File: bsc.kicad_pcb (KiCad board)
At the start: 2 copper layers, 120 x 72 mm, 155 parts, among them IC1 ILD217T, IC2 ILD217T, J1 AVR-ISP-6, J2 Prog, J3 U0TXD silent, J4 Boot, K1 TIANBO-HJR-4102-L, K2 TIANBO-HJR-4102-L, K3 TIANBO-HJR-4102-L, K4 TIANBO-HJR-4102-L, K5 TIANBO-HJR-4102-L, K6 TIANBO-HJR-4102-L, K7 TIANBO-HJR-4102-L, K8 AQY210S, Q1 BSS138, Q10 BC846, Q11 BC846, Q2 BSS138, Q3 BSS138, Q4 BSS138, Q5 BSS138, Q6 BSS138, Q7 BSS138, Q8 BC846, Q9 BC846, U1 LMO78_03-0.5, U10 74HC595, U11 74HC14, U12 74HC165, U2 ESP32WROOM32E16, U3 ATtiny24A-SS, U4 ADuM1201AR, U5 ADuM1201AR, U6 ADuM1201AR, U7 SN65HVD234, U8 SP3485EN, U9 SP3485EN, X1 Conn_S2, X2 Conn_S1, X3 Conn_DI, X4 Conn_SV, X5 Conn_Rel2, X6 Conn_Rel1

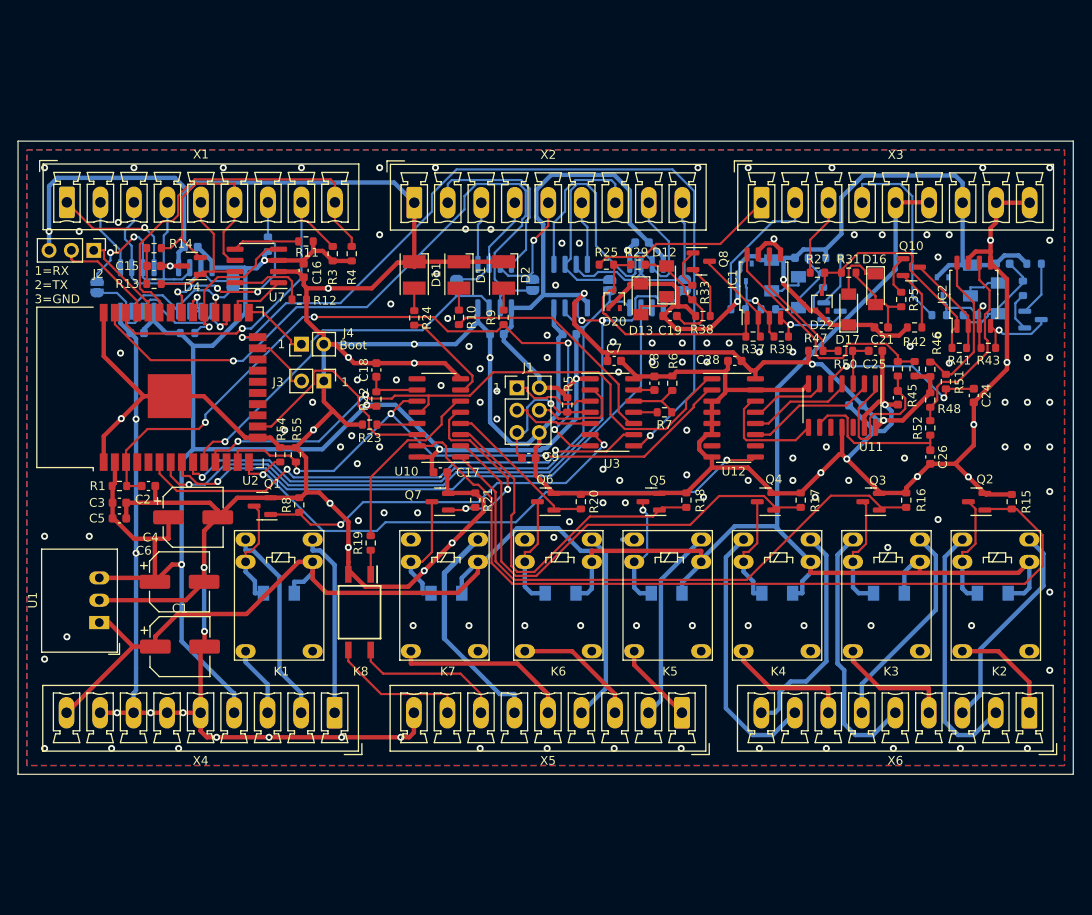
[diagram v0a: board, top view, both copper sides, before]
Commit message: Redesign PCB
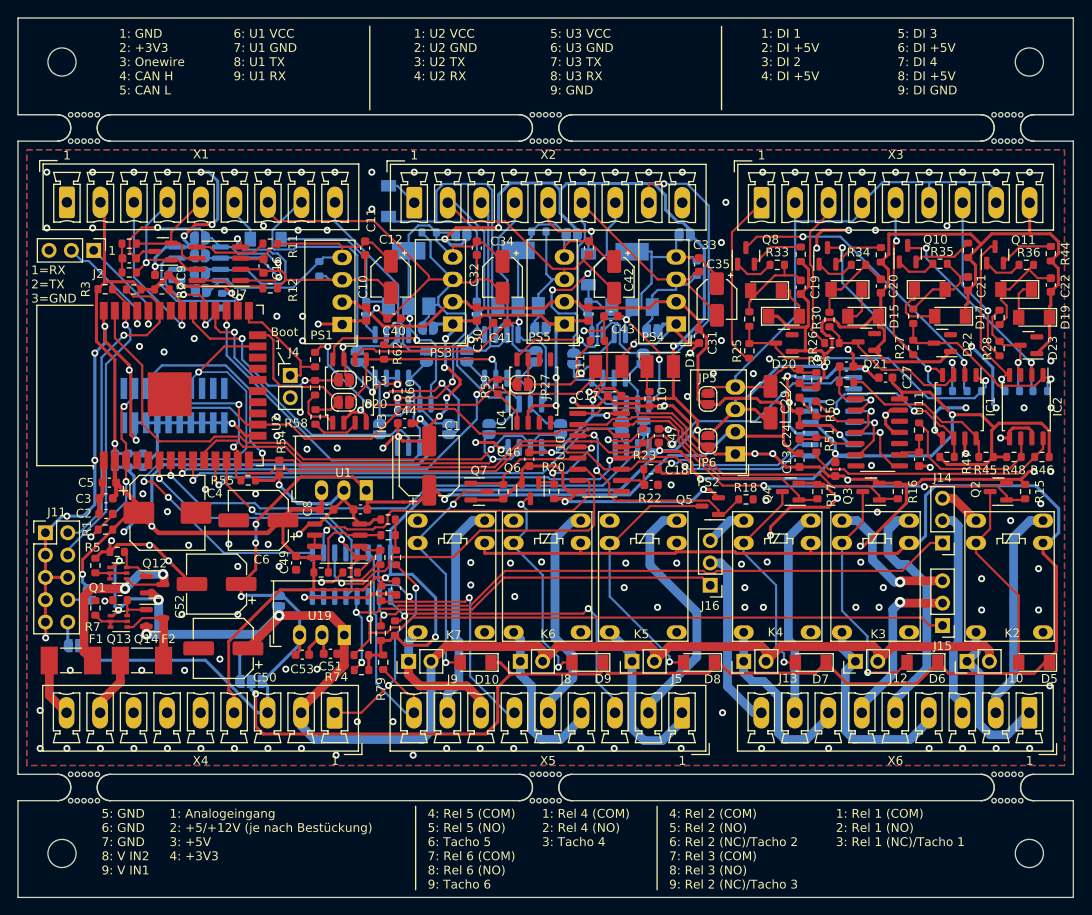
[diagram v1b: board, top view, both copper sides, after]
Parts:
- removed J3: U0TXD silent, Connector_PinHeader_2.54mm:PinHeader_1x02_P2.54mm_Vertical
- removed K1: TIANBO-HJR-4102-L, Relay_THT:Relay_SPDT_HJR-4102
- removed K8: AQY210S, SamacSys_Parts:SOP254P962X275-4N
- removed R9: 180R, Resistor_SMD:R_0603_1608Metric
- removed U3: ATtiny24A-SS, Package_SO:SOIC-14_3.9x8.7mm_P1.27mm
- added C29: 22µ, Capacitor_SMD:CP_Elec_4x5.8, F.Cu at (115.6, 59.7)
- added C30: 100n, Capacitor_SMD:C_0603_1608Metric, F.Cu at (82.2, 49.7)
- added C31: 100n, Capacitor_SMD:C_0603_1608Metric, F.Cu at (107.4, 52.2)
- added C32: 100n, Capacitor_SMD:C_0603_1608Metric, F.Cu at (82.2, 42.2)
- added C33: 100n, Capacitor_SMD:C_0603_1608Metric, F.Cu at (107.4, 44.1)
- added C34: 22µ, Capacitor_SMD:CP_Elec_4x5.8, F.Cu at (85.1, 45.5)
- added C35: 22µ, Capacitor_SMD:CP_Elec_4x5.8, F.Cu at (109.5, 48.0)
- added C36: 100n, Capacitor_SMD:C_0603_1608Metric, B.Cu at (69.6, 49.0)
- added C37: 100n, Capacitor_SMD:C_0603_1608Metric, B.Cu at (94.9, 49.0)
- added C38: 100n, Capacitor_SMD:C_0603_1608Metric, F.Cu at (94.9, 49.7)
- added C39: 100n, Capacitor_SMD:C_0603_1608Metric, F.Cu at (94.9, 42.1)
- added C40: 100n, Capacitor_SMD:C_0603_1608Metric, F.Cu at (72.8, 50.2)
- added C41: 100n, Capacitor_SMD:C_0603_1608Metric, F.Cu at (84.8, 50.7)
- added C42: 22µ, Capacitor_SMD:CP_Elec_4x5.8, F.Cu at (97.8, 45.5)
- added C43: 100n, Capacitor_SMD:C_0603_1608Metric, F.Cu at (97.4, 49.9)
- added C44: 100n, Capacitor_SMD:C_0603_1608Metric, F.Cu at (74.0, 62.1)
- added C45: 100n, Capacitor_SMD:C_0603_1608Metric, B.Cu at (82.2, 49.0)
- added C46: 100n, Capacitor_SMD:C_0603_1608Metric, F.Cu at (88.1, 66.2)
- added C47: 100n, Capacitor_SMD:C_0603_1608Metric, F.Cu at (102.9, 63.5)
- added C48: 100n, Capacitor_SMD:C_0603_1608Metric, B.Cu at (42.5, 66.3)
- added C49: 100n, Capacitor_SMD:C_0603_1608Metric, F.Cu at (61.6, 78.0)
- added C50: 100µ, Capacitor_SMD:CP_Elec_6.3x5.9, F.Cu at (53.3, 87.7)
- added C51: 100n, Capacitor_SMD:C_0603_1608Metric, F.Cu at (65.5, 88.3)
- added C52: 100µ, Capacitor_SMD:CP_Elec_6.3x5.9, F.Cu at (52.6, 80.4)
- added C53: 100n, Capacitor_SMD:C_0603_1608Metric, F.Cu at (62.3, 88.4)
- added C54: 100n, Capacitor_SMD:C_0603_1608Metric, B.Cu at (41.0, 66.3)
- added C55: 100n, Capacitor_SMD:C_0603_1608Metric, B.Cu at (44.2, 66.3)
- added C60: 100n, Capacitor_SMD:C_0603_1608Metric, F.Cu at (73.0, 80.8)
- added D24: LL4148, Diode_SMD:D_MiniMELF, B.Cu at (72.1, 36.8)
- added F1: BELFUSE, Fuse:Fuse_0679H, F.Cu at (36.0, 89.1)
- added F2: BELFUSE, Fuse:Fuse_0679H, F.Cu at (44.1, 89.1)
- added H1: MountingHole, MountingHole:MountingHole_3.2mm_M3, F.Cu at (35.0, 21.0)
- added H2: MountingHole, MountingHole:MountingHole_3.2mm_M3, F.Cu at (145.0, 21.0)
- added H3: MountingHole, MountingHole:MountingHole_3.2mm_M3, F.Cu at (145.0, 111.0)
- added H4: MountingHole, MountingHole:MountingHole_3.2mm_M3, F.Cu at (35.0, 111.0)
- added IC3: ILD217T, Package_SO:SOIC-8_5.23x5.23mm_P1.27mm, F.Cu at (67.7, 58.4)
- added IC4: ILD217T, Package_SO:SOIC-8_5.23x5.23mm_P1.27mm, F.Cu at (88.6, 58.4)
- added J10: JP_REL1_COM_12V, Connector_PinHeader_2.54mm:PinHeader_1x02_P2.54mm_Vertical, F.Cu at (137.9, 89.2)
- added J11: Conn_Extension, Connector_PinHeader_2.54mm:PinHeader_2x05_P2.54mm_Vertical, F.Cu at (33.1, 74.5)
- added J12: JP_REL2_COM_12V, Connector_PinHeader_2.54mm:PinHeader_1x02_P2.54mm_Vertical, F.Cu at (125.2, 89.2)
- added J13: JP_REL3_COM_12V, Connector_PinHeader_2.54mm:PinHeader_1x02_P2.54mm_Vertical, F.Cu at (112.5, 89.2)
- added J14: Conn_REL1, Connector_PinHeader_2.54mm:PinHeader_1x03_P2.54mm_Vertical, F.Cu at (135.1, 75.7)
- added J15: Conn_REL2, Connector_PinHeader_2.54mm:PinHeader_1x03_P2.54mm_Vertical, F.Cu at (135.1, 85.1)
- added J16: Conn_REL3, Connector_PinHeader_2.54mm:PinHeader_1x03_P2.54mm_Vertical, F.Cu at (108.7, 80.5)
- added J5: JP_REL4_COM_12V, Connector_PinHeader_2.54mm:PinHeader_1x02_P2.54mm_Vertical, F.Cu at (99.8, 89.2)
- added J8: JP_REL5_COM_12V, Connector_PinHeader_2.54mm:PinHeader_1x02_P2.54mm_Vertical, F.Cu at (87.1, 89.2)
- added J9: JP_REL6_COM_12V, Connector_PinHeader_2.54mm:PinHeader_1x02_P2.54mm_Vertical, F.Cu at (74.4, 89.2)
- added JP10: JP_U1_TX_TXS, Jumper:SolderJumper-2_P1.3mm_Open_RoundedPad1.0x1.5mm, B.Cu at (71.1, 62.7)
- added JP11: JP_U1_RXS_RXO, Jumper:SolderJumper-2_P1.3mm_Open_RoundedPad1.0x1.5mm, B.Cu at (76.5, 54.5)
- added JP12: JP_U1_TXS_TXO, Jumper:SolderJumper-2_P1.3mm_Open_RoundedPad1.0x1.5mm, B.Cu at (68.6, 54.5)
- added JP13: JP_U1_TXEN_TXENS, Jumper:SolderJumper-2_P1.3mm_Open_RoundedPad1.0x1.5mm, F.Cu at (67.1, 57.1)
- added JP14: JP_U2_3V3_VCC, Jumper:SolderJumper-2_P1.3mm_Open_RoundedPad1.0x1.5mm, B.Cu at (93.0, 40.6)
- added JP15: JP_U2_GND_GNDS, Jumper:SolderJumper-2_P1.3mm_Open_RoundedPad1.0x1.5mm, B.Cu at (89.4, 51.3)
- added JP16: JP_U2_RX_RXS, Jumper:SolderJumper-2_P1.3mm_Open_RoundedPad1.0x1.5mm, B.Cu at (91.7, 62.7)
- added JP17: JP_U2_TX_TXS, Jumper:SolderJumper-2_P1.3mm_Open_RoundedPad1.0x1.5mm, B.Cu at (83.6, 62.7)
- added JP18: JP_U2_RXS_RXO, Jumper:SolderJumper-2_P1.3mm_Open_RoundedPad1.0x1.5mm, B.Cu at (88.9, 54.5)
- added JP19: JP_U2_TXS_TXO, Jumper:SolderJumper-2_P1.3mm_Open_RoundedPad1.0x1.5mm, B.Cu at (81.0, 54.5)
- added JP20: JP_U2_TXEN_TXENS, Jumper:SolderJumper-2_P1.3mm_Open_RoundedPad1.0x1.5mm, F.Cu at (67.1, 59.7)
- added JP21: JP_U3_3V3_VCC, Jumper:SolderJumper-2_P1.3mm_Open_RoundedPad1.0x1.5mm, B.Cu at (105.8, 40.6)
- added JP22: JP_U3_GND_GNDS, Jumper:SolderJumper-2_P1.3mm_Open_RoundedPad1.0x1.5mm, B.Cu at (102.1, 51.6)
- added JP23: JP_U3_RX_RXS, Jumper:SolderJumper-2_P1.3mm_Open_RoundedPad1.0x1.5mm, B.Cu at (101.2, 62.4)
- added JP24: JP_U3_TX_TXS, Jumper:SolderJumper-2_P1.3mm_Open_RoundedPad1.0x1.5mm, B.Cu at (98.7, 62.4)
- added JP25: JP_U3_RXS_RXO, Jumper:SolderJumper-2_P1.3mm_Open_RoundedPad1.0x1.5mm, B.Cu at (101.1, 54.7)
- added JP26: JP_U3_TXS_TXO, Jumper:SolderJumper-2_P1.3mm_Open_RoundedPad1.0x1.5mm, B.Cu at (93.2, 54.7)
- added JP27: JP_U3_TXEN_TXENS, Jumper:SolderJumper-2_P1.3mm_Open_RoundedPad1.0x1.5mm, F.Cu at (87.4, 57.7)
- added JP28: 12V_5V, Jumper:SolderJumper-2_P1.3mm_Open_RoundedPad1.0x1.5mm, B.Cu at (59.6, 82.3)
- added JP29: JP_REL_VCC, Jumper:SolderJumper-3_P1.3mm_Open_RoundedPad1.0x1.5mm, B.Cu at (56.5, 91.4)
- added JP30: JP_EXT_5V, Jumper:SolderJumper-2_P1.3mm_Open_RoundedPad1.0x1.5mm, B.Cu at (36.4, 87.4)
- added JP31: JP_EXT_3V3, Jumper:SolderJumper-2_P1.3mm_Open_RoundedPad1.0x1.5mm, B.Cu at (38.1, 81.5)
- added JP7: JP_U1_3V3_VCC, Jumper:SolderJumper-2_P1.3mm_Open_RoundedPad1.0x1.5mm, B.Cu at (80.4, 40.6)
- added JP8: JP_U1_GND_GNDS, Jumper:SolderJumper-2_P1.3mm_Open_RoundedPad1.0x1.5mm, B.Cu at (76.6, 51.3)
- added JP9: JP_U1_RX_RXS, Jumper:SolderJumper-2_P1.3mm_Open_RoundedPad1.0x1.5mm, B.Cu at (79.0, 62.7)
- added PS1: 1S4E_0503S1U, custom_th:Converter_DCDC_GAPTEC_1S4E_S1U, F.Cu at (66.9, 50.9)
- added PS2: TEA 1-0505, Converter_DCDC:Converter_DCDC_Murata_MEE1SxxxxSC_THT, F.Cu at (111.6, 65.6)
- added PS3: 1S4E_0503S1U, custom_th:Converter_DCDC_GAPTEC_1S4E_S1U, F.Cu at (79.4, 50.8)
- added PS4: 1S4E_0503S1U, custom_th:Converter_DCDC_GAPTEC_1S4E_S1U, F.Cu at (104.8, 50.8)
- added PS5: 1S4E_0503S1U, custom_th:Converter_DCDC_GAPTEC_1S4E_S1U, F.Cu at (92.1, 50.8)
- added Q12: IRLML2244, Package_TO_SOT_SMD:SOT-23, F.Cu at (45.5, 80.4)
- added Q13: BC857BS, Package_TO_SOT_SMD:SOT-363_SC-70-6, F.Cu at (41.5, 84.6)
- added Q14: IRLML2244, Package_TO_SOT_SMD:SOT-23, F.Cu at (45.5, 84.2)
- added R56: n.b., Resistor_SMD:R_0603_1608Metric, F.Cu at (120.8, 57.1)
- added R57: 330R, Resistor_SMD:R_0603_1608Metric, F.Cu at (63.8, 58.0)
- added R58: 330R, Resistor_SMD:R_0603_1608Metric, F.Cu at (63.8, 61.4)
- added R59: 330R, Resistor_SMD:R_0603_1608Metric, F.Cu at (84.6, 57.9)
- added R60: 2k2, Resistor_SMD:R_0603_1608Metric, F.Cu at (73.2, 58.4)
- added R61: 2k2, Resistor_SMD:R_0603_1608Metric, F.Cu at (95.9, 52.7)
- added R62: 2k2, Resistor_SMD:R_0603_1608Metric, F.Cu at (71.6, 54.0)
- added R63: n.b., Resistor_SMD:R_0603_1608Metric, B.Cu at (76.7, 40.4)
- added R64: n.b., Resistor_SMD:R_0603_1608Metric, B.Cu at (107.2, 44.5)
- added R65: n.b., Resistor_SMD:R_0603_1608Metric, B.Cu at (89.2, 40.3)
- added R66: 10k, Resistor_SMD:R_0603_1608Metric, F.Cu at (73.0, 77.3)
- added R67: 2k4, Resistor_SMD:R_0603_1608Metric, F.Cu at (72.1, 73.0)
- added R68: 470R, Resistor_SMD:R_0603_1608Metric, F.Cu at (72.1, 74.8)
- added R69: 47k, Resistor_SMD:R_0603_1608Metric, F.Cu at (64.5, 79.0)
- added R70: 20k, Resistor_SMD:R_0603_1608Metric, F.Cu at (67.8, 79.0)
- added R71: 10k, Resistor_SMD:R_0603_1608Metric, F.Cu at (71.2, 77.3)
- added R74: 4k7, Resistor_SMD:R_0603_1608Metric, F.Cu at (69.1, 90.1)
- added R75: 4k7, Resistor_SMD:R_0603_1608Metric, F.Cu at (69.0, 88.4)
- added R76: 4k7, Resistor_SMD:R_0603_1608Metric, F.Cu at (71.2, 86.0)
- added R77: 4k7, Resistor_SMD:R_0603_1608Metric, F.Cu at (72.9, 85.4)
- added R78: 4k7, Resistor_SMD:R_0603_1608Metric, F.Cu at (71.3, 81.4)
- added R79: 4k7, Resistor_SMD:R_0603_1608Metric, F.Cu at (71.5, 89.3)
- added U13: ADuM1201AR, Package_SO:SOIC-8_3.9x4.9mm_P1.27mm, B.Cu at (50.5, 43.9)
- added U14: NCP1117-3.3_SOT223, Package_TO_SOT_SMD:SOT-223-3_TabPin2, B.Cu at (74.4, 45.6)
- added U15: NCP1117-3.3_SOT223, Package_TO_SOT_SMD:SOT-223-3_TabPin2, B.Cu at (99.8, 45.7)
- added U16: SP3485EN, Package_SO:SOIC-8_3.9x4.9mm_P1.27mm, B.Cu at (85.0, 54.5)
- added U17: NCP1117-3.3_SOT223, Package_TO_SOT_SMD:SOT-223-3_TabPin2, B.Cu at (86.9, 45.6)
- added U18: TS912, Package_SO:SO-8_3.9x4.9mm_P1.27mm, F.Cu at (66.3, 75.4)
- added U19: LMO78_05-0.5, custom_th:Converter_DCDC_RECOM_R-78E-1.0, F.Cu at (64.4, 83.6)
- added U20: HC 151, Package_SO:SOIC-16_3.9x9.9mm_P1.27mm, B.Cu at (67.9, 79.3)
- added mouse-bite-3mm-slot: VAL**, mouse_bites:mouse-bite-3mm-slot, F.Cu at (142.5, 28.5)
- added mouse-bite-3mm-slot: VAL**, mouse_bites:mouse-bite-3mm-slot, F.Cu at (142.5, 103.5)
- added mouse-bite-3mm-slot: VAL**, mouse_bites:mouse-bite-3mm-slot, F.Cu at (37.5, 103.5)
- added mouse-bite-3mm-slot: VAL**, mouse_bites:mouse-bite-3mm-slot, F.Cu at (37.5, 28.5)
- added mouse-bite-3mm-slot: VAL**, mouse_bites:mouse-bite-3mm-slot, F.Cu at (90.0, 103.5)
- added mouse-bite-3mm-slot: VAL**, mouse_bites:mouse-bite-3mm-slot, F.Cu at (90.0, 28.5)
- C1: value 10µ -> 100µ
- C10, C11, C13, C14, C20, C22, C27, D10, D14, D15, D18, D19, D5, D6, D7, D8, D9, Q11, Q9, R2, R26, R28, R30, R32, R34, R36, R40, R44: moved to F.Cu
- C12: value 100n -> 22µ; footprint Capacitor_SMD:C_0603_1608Metric -> Capacitor_SMD:CP_Elec_4x5.8; moved to F.Cu
- C15, C16, C5, C8: value 100nF -> 100n
- C4: value 22µ -> 470µ/6,3V; footprint Capacitor_SMD:CP_Elec_6.3x5.9 -> Capacitor_SMD:CP_Elec_8x10
- C6: value 22µ -> 100µ
- D2: value LED3 -> LL4148; footprint LED_SMD:LED_PLCC-2 -> Diode_SMD:D_MiniMELF; moved to B.Cu
- D20, D22: footprint Package_TO_SOT_SMD:SOT-323_SC-70 -> Package_TO_SOT_SMD:SOT-23
- D21, D23: footprint Package_TO_SOT_SMD:SOT-323_SC-70 -> Package_TO_SOT_SMD:SOT-23; moved to F.Cu
- J1: value AVR-ISP-6 -> Conn_JTAG_ESP; footprint Connector_PinHeader_2.54mm:PinHeader_2x03_P2.54mm_Vertical -> Connector_PinHeader_1.27mm:PinHeader_2x10_P1.27mm_Vertical_SMD; moved to B.Cu
- JP1: value O_U2RXD -> CAN_VCC
- JP2: value O_U2TXD -> CAN_GND
- JP3: value O_SU1RXD -> CAN_RC
- JP4: value O_SU1TXD -> CAN_TX
- JP5: value O_SU2RXD -> DI_VCC; moved to F.Cu
- JP6: value O_SU2TXD -> DI_GND; moved to F.Cu
- Q1: value BSS138 -> BC857BS; footprint Package_TO_SOT_SMD:SOT-23 -> Package_TO_SOT_SMD:SOT-363_SC-70-6
- Q5, Q6, Q7: value BSS138 -> IRLML 2502
- R19: value 180R -> n.b.; moved to B.Cu
- R37, R39, R41, R43, U12: moved to B.Cu
- R53, R54: value 10k -> n.b.
- R8: value 100k -> 10k
- U1: footprint Converter_DCDC:Converter_DCDC_RECOM_R-78E-0.5_THT -> custom_th:Converter_DCDC_RECOM_R-78E-1.0
- moved R7 68.4 mm to (38.8, 83.1), turned to 90 degrees
- moved R6 66.0 mm to (41.3, 76.7), turned to 180 degrees
- moved R5 56.7 mm to (38.8, 78.3), turned to 90 degrees
- moved JP3 55.1 mm to (50.7, 45.0), turned to 0 degrees
- moved JP4 46.7 mm to (50.7, 43.0), turned to 0 degrees
- moved C9 46.6 mm to (46.4, 45.2), turned to 180 degrees
- moved D3 40.3 mm to (58.2, 41.1)
- moved C8 39.9 mm to (65.1, 71.9), turned to 0 degrees
- moved J1 39.0 mm to (47.8, 60.1), turned to -90 degrees
- moved U4 35.1 mm to (75.1, 62.4)
- moved C1 35.0 mm to (76.8, 66.9), turned to 90 degrees
- moved C18 33.9 mm to (102.0, 69.1), turned to 0 degrees
- moved JP6 33.7 mm to (108.5, 64.1)
- moved C7 33.4 mm to (68.9, 71.9), turned to 180 degrees
- moved U1 32.8 mm to (66.9, 67.1), turned to 0 degrees
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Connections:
- net /INPUT/IO_DATA_IN_DS renamed /INPUT/IO_DATA_OUT
- net /OUTPUT/DATA_OUT renamed /OUTPUT/IO_DATA_IN
- C10 pad 1: +3V3 -> +5V
- C11 pad 1: +3V3 -> /CAN_VCC
- C11 pad 2: GND -> /CAN_GND
- C12 pad 1: +3V3 -> /CAN_VCC
- C12 pad 2: GND -> /CAN_GND
- C13 pad 1: +3V3 -> +5V
- C14 pad 1: +3V3 -> /INPUT/5V_1
- C14 pad 2: GND -> GND1
- C15 pad 2: GND -> /CAN_GND
- C16 pad 1: +3V3 -> /CAN_VCC
- C16 pad 2: GND -> /CAN_GND
- C7 pad 1: +3V3 -> +5V
- C8 pad 1: GND -> +3V3
- C8 pad 2: Net-(C8-Pad2) -> GND
- C9 pad 1: /AVR_RST -> +3V3
- D1 pad 1: GND -> Net-(D1-Pad1)
- D1 pad 2: Net-(D1-Pad2) -> +3V3
- D10 pad 1: +5V -> /OUTPUT/VCC_REL
- D2 pad 1: GND -> Net-(C37-Pad1)
- D2 pad 2: Net-(D2-Pad2) -> /serial/U3_VCC_e
- D3 pad 1: +5V -> Net-(C36-Pad1)
- D3 pad 2: Net-(D3-Pad2) -> /U1_VCC_e
- D4 pad 3: GND -> /CAN_GND
- D5 pad 1: +5V -> /OUTPUT/VCC_REL
- D6 pad 1: +5V -> /OUTPUT/VCC_REL
- D7 pad 1: +5V -> /OUTPUT/VCC_REL
- D8 pad 1: +5V -> /OUTPUT/VCC_REL
- D9 pad 1: +5V -> /OUTPUT/VCC_REL
- J1 pad 1: /AVR_MISO -> unconnected-(J1-Pad1)
- J1 pad 2: +3V3 -> unconnected-(J1-Pad2)
- J1 pad 3: /AVR_SCK -> /RST_ESP
- J1 pad 4: /AVR_MOSI -> GND
- J1 pad 5: /AVR_RST -> /H_MISO
- J4 pad 1: Net-(J4-Pad1) -> /LED1
- JP1 pad 1: /U1RX -> +3V3
- JP1 pad 2: /U1RX_O -> /CAN_VCC
- JP2 pad 1: /U1TX -> GND
- JP2 pad 2: /U1TX_O -> /CAN_GND
- JP3 pad 1: /U3RX -> /CAN_Rx
- JP3 pad 2: /U3RX_O -> /CAN_Rx_s
- JP4 pad 1: /U3TX -> /CAN_Tx
- JP4 pad 2: /U3TX_O -> /CAN_Tx_s
- JP5 pad 1: /U2RX -> +5V
- JP5 pad 2: /U2RX_O -> /INPUT/5V_1
- JP6 pad 1: /U2TX -> GND
- JP6 pad 2: /U2TX_O -> GND1
- K2 pad 5: +5V -> /OUTPUT/VCC_REL
- K3 pad 5: +5V -> /OUTPUT/VCC_REL
- K4 pad 5: +5V -> /OUTPUT/VCC_REL
- K5 pad 5: +5V -> /OUTPUT/VCC_REL
- K6 pad 5: +5V -> /OUTPUT/VCC_REL
- K7 pad 5: +5V -> /OUTPUT/VCC_REL
- Q1 pad 1: Net-(Q1-Pad1) -> Net-(F1-Pad2)
- Q1 pad 2: GND -> Net-(Q1-Pad2)
- Q1 pad 3: Net-(D3-Pad2) -> Net-(Q1-Pad3)
- R1 pad 1: +3V3 -> /RST_ESP
- R1 pad 2: /RST_ESP -> +3V3
- R10 pad 1: Net-(D1-Pad2) -> Net-(D1-Pad1)
- R10 pad 2: Net-(R10-Pad2) -> GND
- R11 pad 1: +3V3 -> /CAN_VCC
- R12 pad 1: GND -> /CAN_GND
- R19 pad 1: Net-(K8-Pad1) -> /CAN_GND
- R19 pad 2: /OUTPUT/DO1 -> /CAN_VCC
- R2 pad 1: +3V3 -> /onewire
- R2 pad 2: /onewire -> +3V3
- R24 pad 2: Net-(R24-Pad2) -> /LED1
- R5 pad 1: +3V3 -> Net-(Q1-Pad2)
- R5 pad 2: /AVR_RST -> GND
- R6 pad 1: GND -> Net-(Q1-Pad3)
- R6 pad 2: Net-(R6-Pad2) -> GND
- R7 pad 1: Net-(R6-Pad2) -> Net-(Q13-Pad2)
- R7 pad 2: Net-(R7-Pad2) -> GND
- R8 pad 1: Net-(Q1-Pad1) -> Net-(Q13-Pad3)
- U10 pad 6: /OUTPUT/DO1 -> /OUTPUT/T_ADDR0
- U10 pad 7: Net-(R24-Pad2) -> /OUTPUT/T_ADDR1
- U12 pad 4: GND -> +3V3
- U2 pad 12: Net-(J11-Pad9) -> /TACHO
- U2 pad 23: Net-(J3-Pad2) -> /T_ADDR2
- U2 pad 24: /WDT_TRIG_ESP_OUT -> /U2RXTX_EN
- U2 pad 25: Net-(J4-Pad1) -> /LED1
- U2 pad 6: /WDT_TRIG__ESP_IN -> /AI1d
- U4 pad 6: /U1TX_O -> /serial/U1TX_S
- U4 pad 7: /U1RX_O -> /serial/U1RX_S
- U4 pad 8: /U1_VCC -> /serial/U1_VCC
- U5 pad 5: /U3_GND -> /serial/U3_GND
- U5 pad 6: /U3TX_O -> /serial/U3TX_S
- U5 pad 7: /U3RX_O -> /serial/U3RX_S
- U5 pad 8: /U3_VCC -> /serial/U3_VCC
- U6 pad 5: /U2_GND -> /serial/U2_GND
- U6 pad 6: /U2TX_O -> /serial/U2TX_S
- U6 pad 7: /U2RX_O -> /serial/U2RX_S
- U6 pad 8: /U2_VCC -> /serial/U2_VCC
- U7 pad 1: /CAN_Tx -> /CAN_Tx_s
- U7 pad 2: GND -> /CAN_GND
- U7 pad 3: +3V3 -> /CAN_VCC
- U7 pad 4: /CAN_Rx -> /CAN_Rx_s
- U8 pad 1: /U1RX -> /serial/U1RX_S
- U8 pad 2: /U1RXTX_EN -> /serial/U1RXTX_ENs
- U8 pad 3: /U1RXTX_EN -> /serial/U1RXTX_ENs
- U8 pad 4: /U1TX -> /serial/U1TX_S
- U8 pad 5: GND -> /U1_GND
- U8 pad 8: +3V3 -> /serial/U1_VCC
- U9 pad 1: /U3RX -> /serial/U3RX_S
- U9 pad 2: /U3RXTX_EN -> /serial/U3RXTX_ENs
- U9 pad 3: /U3RXTX_EN -> /serial/U3RXTX_ENs
- U9 pad 4: /U3TX -> /serial/U3TX_S
- U9 pad 5: GND -> /serial/U3_GND
- U9 pad 6: /U3RX_O -> /serial/U3RX_O
- U9 pad 7: /U3TX_O -> /serial/U3TX_O
- U9 pad 8: +3V3 -> /serial/U3_VCC
- X1 pad 1: /U1_VCC -> GND
- X1 pad 2: /U1_GND -> +3V3
- X1 pad 3: /U1TX_O -> /onewire
- X1 pad 4: /U1RX_O -> /CAN_H
- X1 pad 5: /CAN_H -> /CAN_L
- X1 pad 6: /CAN_L -> /U1_VCC_e
- X1 pad 7: /onewire -> /U1_GND
- X1 pad 8: /SCL -> /U1TX_O
- X1 pad 9: /SDA -> /U1RX_O
- X2 pad 1: GND -> /serial/U2_VCC_e
- X2 pad 2: /U2_VCC -> /serial/U2_GND
- X2 pad 3: /U2_GND -> /serial/U2TX_O
- X2 pad 4: /U2TX_O -> /serial/U2RX_O
- X2 pad 5: /U2RX_O -> /serial/U3_VCC_e
- X2 pad 6: /U3_VCC -> /serial/U3_GND
- X2 pad 7: /U3_GND -> /serial/U3TX_O
- X2 pad 8: /U3TX_O -> /serial/U3RX_O
- X2 pad 9: /U3RX_O -> GND
- X3 pad 2: /INPUT/DI2_P -> /INPUT/5V_1
- X3 pad 3: /INPUT/DI3_P -> /INPUT/DI2_P
- X3 pad 4: /INPUT/DI4_P -> /INPUT/5V_1
- X3 pad 5: +5V -> /INPUT/DI3_P
- X3 pad 6: +5V -> /INPUT/5V_1
- X3 pad 7: GND1 -> /INPUT/DI4_P
- X3 pad 8: GND -> /INPUT/5V_1
- X3 pad 9: GND -> GND1
- X4 pad 1: /REL0_NO -> /AI1
- X4 pad 2: /REL0_NC -> V_IN
- X4 pad 3: /REL0_COM -> +5V
- X4 pad 8: GND -> V_IN2
- X4 pad 9: +5V -> V_IN1
- X5 pad 3: /OUTPUT/REL5_COM -> /OUTPUT/TACHO4
- X5 pad 4: /OUTPUT/REL5_NO -> /OUTPUT/REL5_COM
- X5 pad 5: /OUTPUT/REL6_COM -> /OUTPUT/REL5_NO
- X5 pad 6: /OUTPUT/REL6_NO -> /OUTPUT/TACHO5
- X5 pad 7: /OUTPUT/DO1_1 -> /OUTPUT/REL6_COM
- X5 pad 8: /OUTPUT/DO1_2 -> /OUTPUT/REL6_NO
- X5 pad 9: GND -> /OUTPUT/TACHO6
- X6 pad 2: /OUTPUT/REL1_NC -> /OUTPUT/REL1_NO
- X6 pad 3: /OUTPUT/REL1_NO -> /OUTPUT/REL1_NC_TACHO
- X6 pad 5: /OUTPUT/REL2_NC -> /OUTPUT/REL2_NO
- X6 pad 6: /OUTPUT/REL2_NO -> /OUTPUT/REL2_NC_TACHO
- X6 pad 8: /OUTPUT/REL3_NC -> /OUTPUT/REL3_NO
- X6 pad 9: /OUTPUT/REL3_NO -> /OUTPUT/REL3_NC_TACHO
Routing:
- net /OUTPUT/VCC_REL: track 0.00 -> 207.6 mm, vias 0 -> 1
- net V_IN: track 0.00 -> 170.5 mm, vias 0 -> 5
- net GND: track 617.5 -> 477.9 mm, vias 151 -> 194
- net +3V3: track 307.1 -> 444.3 mm, vias 8 -> 19
- net /WDT_TRIG_ESP_OUT: track 95.5 -> 0.00 mm, vias 2 -> 0
- net /serial/U2_GND: track 0.00 -> 84.7 mm, vias 0 -> 1
- net /OUTPUT/TACHO1: track 0.00 -> 79.2 mm, vias 0 -> 2
- net /OUTPUT/TACHO2: track 0.00 -> 73.7 mm, vias 0 -> 1
- net /U1_GND: track 8.38 -> 81.2 mm, vias 0 -> 3
- net /INPUT/5V_1: track 0.00 -> 68.0 mm
- net /serial/U3_GND: track 0.00 -> 67.1 mm, vias 0 -> 2
- net /WDT_TRIG__ESP_IN: track 60.0 -> 0.00 mm, vias 2 -> 0
- net /serial/U2_VCC: track 0.00 -> 60.0 mm, vias 0 -> 1
- net /T_ADDR2: track 0.00 -> 57.9 mm, vias 0 -> 3
- net /serial/U3_VCC: track 0.00 -> 57.1 mm, vias 0 -> 3
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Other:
- board size 120 x 72 mm -> 120 x 100 mm
- board text added: "(Frontside) JP5: +5V -> DI_VCC JP6: GND -> DI_GND"
- board text added: "1: Analogeingang 2: +5/+12V (je nach Bestückung) 3: +5V 4: +3V3"
- board text added: "1: DI 1 2: DI +5V 3: DI 2 4: DI +5V"
- board text added: "1: GND 2: +3V3 3: Onewire 4: CAN H 5: CAN L"
- board text added: "1: Rel 1 (COM) 2: Rel 1 (NO) 3: Rel 1 (NC)/Tacho 1"
- board text added: "1: Rel 4 (COM) 2: Rel 4 (NO) 3: Tacho 4"
- board text added: "1: U2 VCC 2: U2 GND 3: U2 TX 4: U2 RX"
- board text added: "4: Rel 2 (COM) 5: Rel 2 (NO) 6: Rel 2 (NC)/Tacho 2 7: Rel 3 (COM) 8: Rel 3 (NO) 9: Rel 2 (NC)/Tacho 3"
- board text added: "4: Rel 5 (COM) 5: Rel 5 (NO) 6: Tacho 5 7: Rel 6 (COM) 8: Rel 6 (NO) 9: Tacho 6"
- board text added: "5: DI 3 6: DI +5V 7: DI 4 8: DI +5V 9: DI GND"
- board text added: "5: GND 6: GND 7: GND 8: V IN2 9: V IN1"
- board text added: "5: U3 VCC 6: U3 GND 7: U3 TX 8: U3 RX 9: GND"
- board text added: "6: U1 VCC 7: U1 GND 8: U1 TX 9: U1 RX"
- board text added: "Battery safety controller V2.0 github.com/shining-man/bsc_fw created by T. Himmler 2022"
- board text added: "JP1: CAN VCC JP2: CAN GND JP3: CAN RX JP4: CAN TX"
- board text added: "JP28: V_IN -> +5V"
- board text added: "JP29 VCC REL: 1-2: +5V | 2-3: V_IN"
- board text added: "JP30: 5V to Ext.-Port JP31: 3V3 to Ext.-Port"
- board text added: "U1|U2|U3| JP 07|14|21|3V3->Ux_VCC JP 08|15|22|GND->Ux_GND JP 09|16|23|UxRX->UxRX_S JP 10|17|24|UxTX->UxTX_S JP 11|18|25|UxRX_S->UxRX_O JP 12|19|26|UxTX_S->UxTX_O JP 13|20|27|UxRXTX_EN->UxRXTX_ENs"
- board text removed: "Battery safety controller (BSC) V1.0 (c) T. Himmler 2022"
- board text removed: "JP1: Serial 1, RXD JP2: Serial 1, TXD JP3: Serial 2, RXD JP4: Serial 2, TXD JP5: Serial 3, RXD JP6: Serial 3, TXD"
